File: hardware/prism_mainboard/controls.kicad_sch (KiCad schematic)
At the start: 1 part, among them U3 PEC16-4220F-S0024

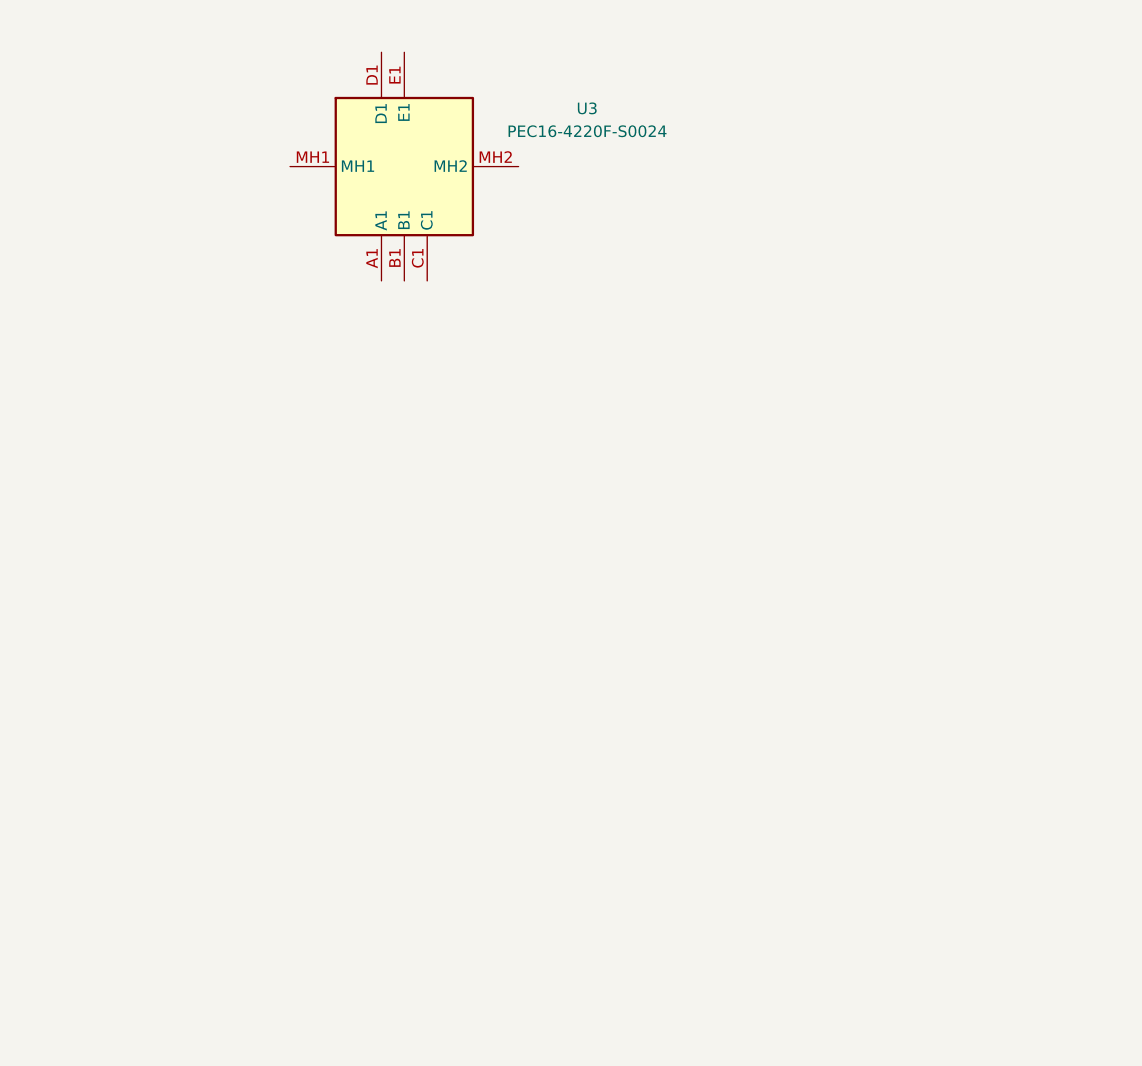
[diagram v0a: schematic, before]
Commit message: Updates
Mostly Schematic updates, nothing too big. Added a few datasheets
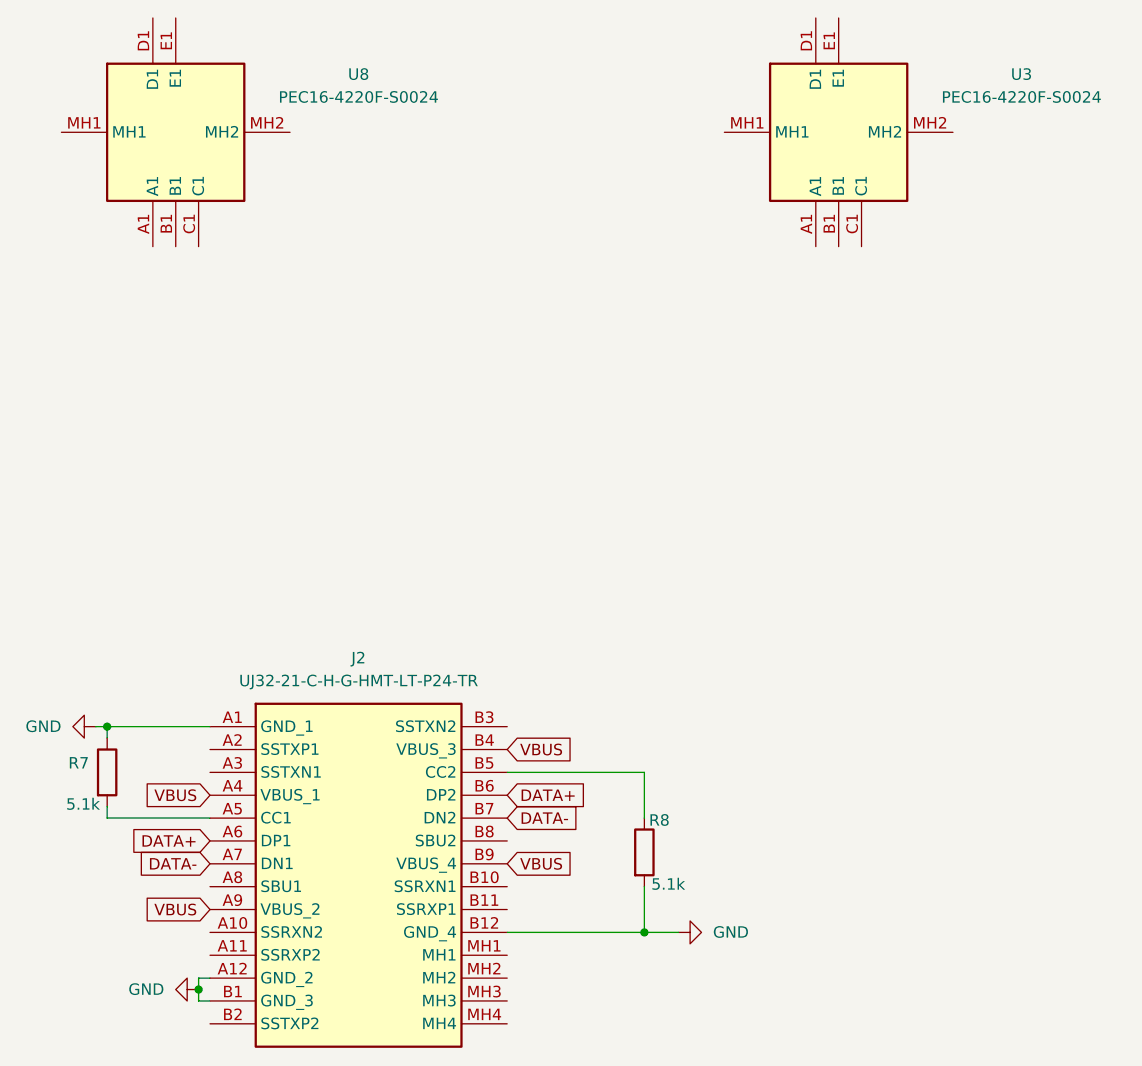
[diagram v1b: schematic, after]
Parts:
- added J2: UJ32-21-C-H-G-HMT-LT-P24-TR, UJ3221CHGHMTLTP24TR, symbol SamacSys:UJ32-21-C-H-G-HMT-LT-P24-TR
- added R7, R8: 5.1k, symbol Device:R
- added U8: PEC16-4220F-S0024, PEC164120FS0012, symbol SamacSys:PEC16-4220F-S0024
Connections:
- new net: J2.A5 (CC1), R7.2
- new net: J2.B5 (CC2), R8.1
- new net DATA+: J2.A6 (DP1), J2.B6 (DP2)
- new net DATA-: J2.A7 (DN1), J2.B7 (DN2)
- new net GND: J2.A1 (GND_1), J2.A12 (GND_2), J2.B1 (GND_3), J2.B12 (GND_4), R7.1, R8.2
- new net VBUS: J2.A4 (VBUS_1), J2.A9 (VBUS_2), J2.B4 (VBUS_3), J2.B9 (VBUS_4)
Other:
- moved on the sheet: U3
